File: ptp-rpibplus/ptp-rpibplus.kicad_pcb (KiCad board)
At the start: 2 copper layers, 65.5 x 56.6 mm, 9 parts, among them J1 RASPI_B+, J2 MODULE_HEADER, J3 MODULE_HEADER

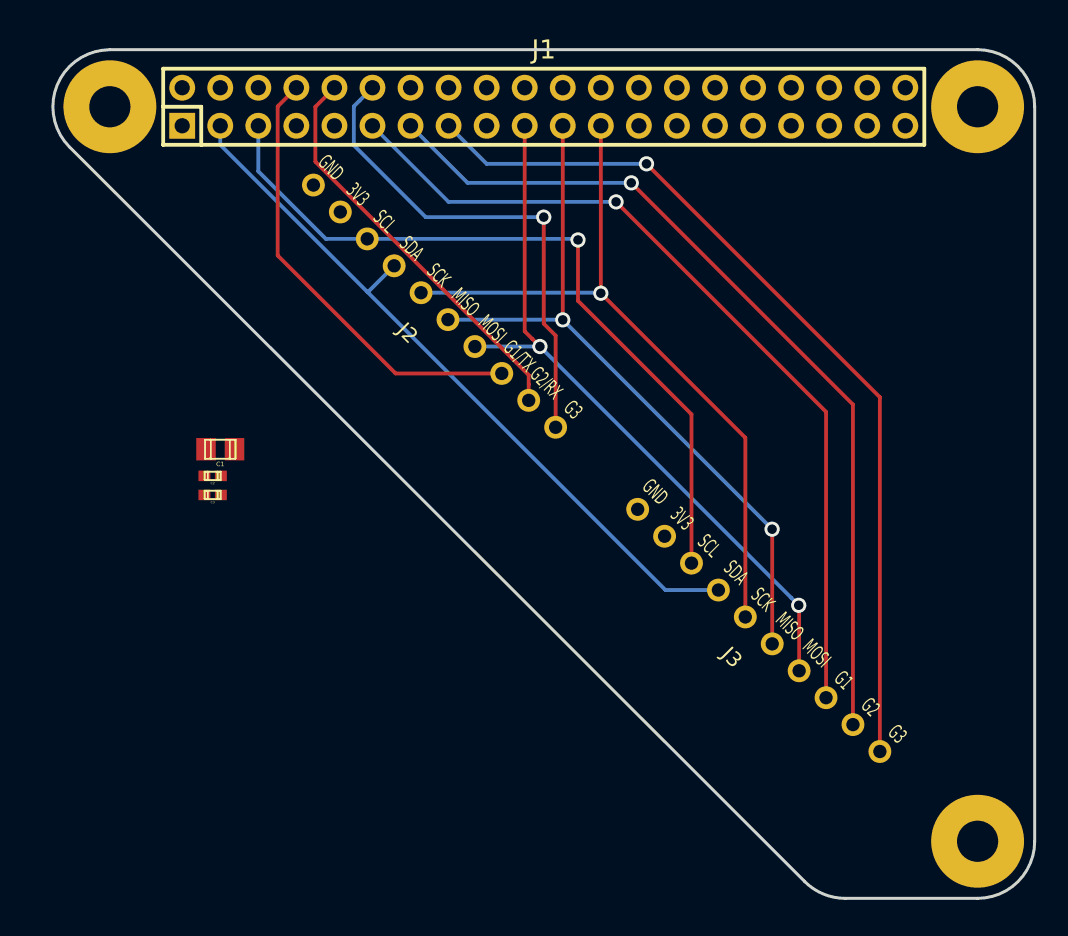
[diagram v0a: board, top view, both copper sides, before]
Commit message: really really close
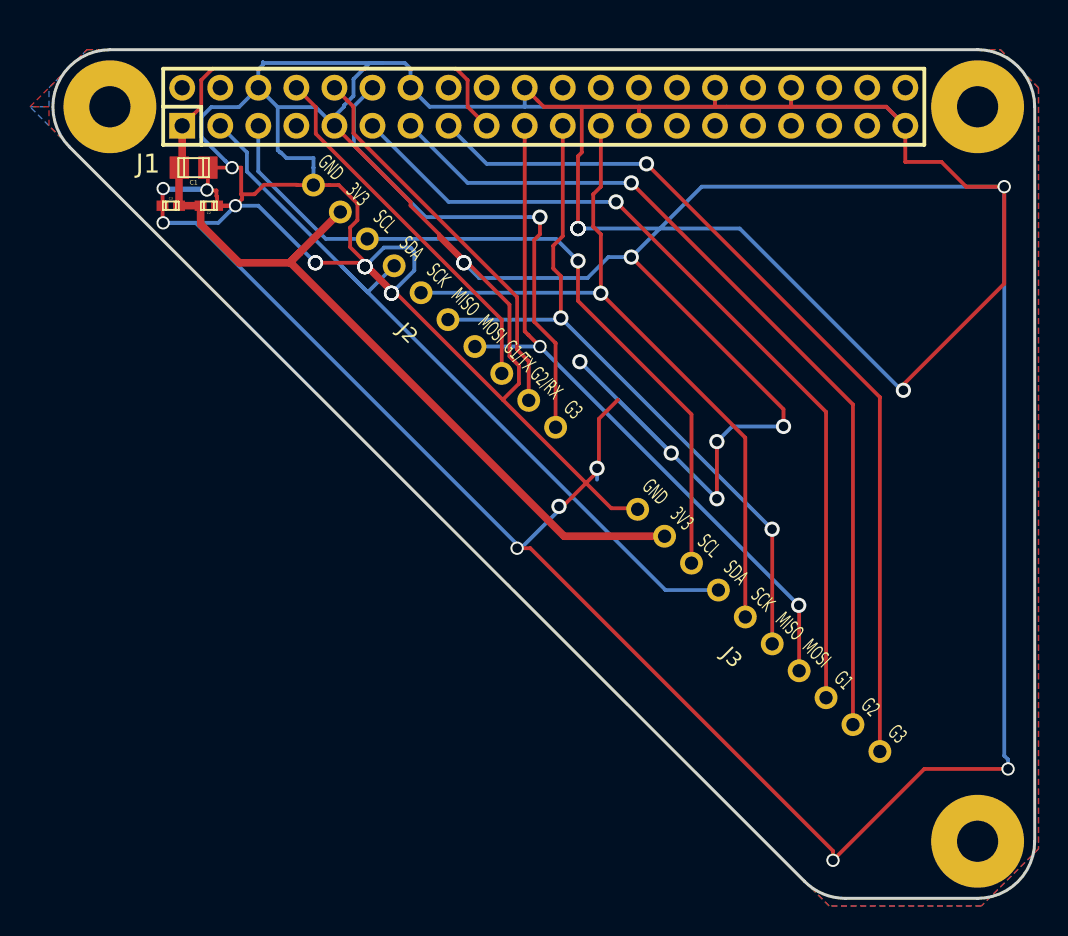
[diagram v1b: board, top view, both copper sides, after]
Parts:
- moved C3 19.5 mm to (102.1, 86.6), turned to 0 degrees
- moved C1 18.9 mm to (103.6, 84.1)
- moved C2 18.0 mm to (104.6, 86.6)
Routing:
- net GND: track 0.00 -> 514.4 mm, vias 0 -> 32
- net 3V3: track 0.00 -> 78.9 mm
- net /A_G1/TX: track 29.9 -> 24.7 mm
- net /SDA: track 49.3 -> 51.7 mm
- net /A_G2/RX: track 27.3 -> 26.2 mm
- net /SCL: track 51.0 -> 50.2 mm
- added copper zone on B.Cu, net GND
- added copper zone on F.Cu, net GND
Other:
- net class Default: via_dia 0.889 -> 1.016
- rule pad_to_mask_clearance: 0 -> 0.0762
- rule via_min_size: 0.889 -> 1.016
